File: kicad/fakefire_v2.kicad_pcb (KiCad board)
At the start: 2 copper layers, 212 x 96 mm, 46 parts, among them J1 Barrel_Jack, J2 Conn_01x03_Female, J3 Left speaker, J4 Right speaker, Q2 IRLB3813PBF, U1 YAAJ_DCDC_StepDown_LM2596, U2 PAM8403_Module, U3 TSOP1838B, U4 DFR0299, U5 Raspberry Pico, U6 4011

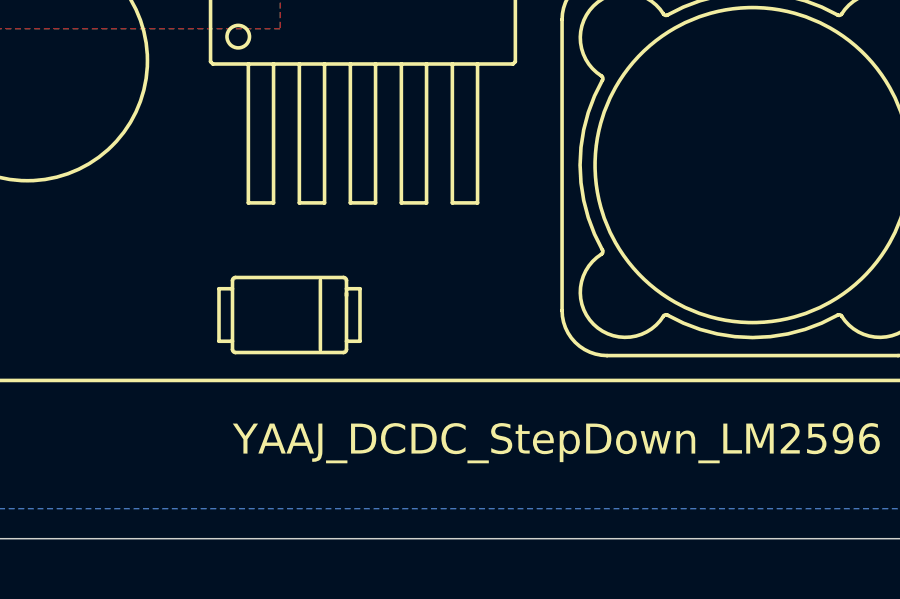
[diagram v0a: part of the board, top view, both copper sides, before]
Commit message: update kicad files, added more infos, comments
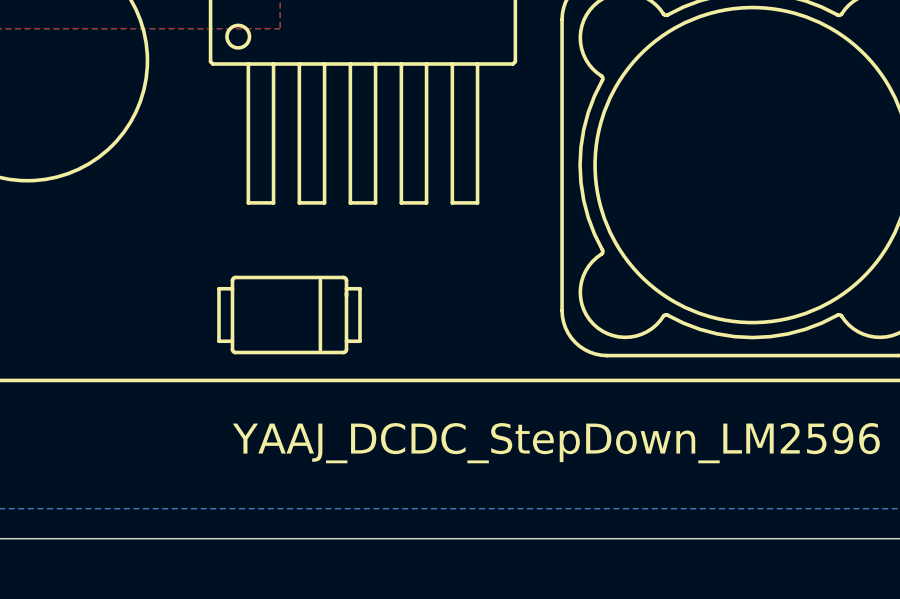
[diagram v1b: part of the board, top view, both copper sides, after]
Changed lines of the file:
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@@
   )
   (paper "A4")
+  (title_block
+    (title "Fakefire Project")
+    (date "2023-02-02")
+    (rev "1")
+    (company "N/A")
+  )
   (layers
     (0 "F.Cu" signal)
@@
     (fp_arc (start 20.467397 7.585796) (mid 20.906738 6.525137) (end 21.967397 6.085796) (layer "F.SilkS") (width 0.12))
     (fp_arc (start 21.781131 9.46601) (mid 21.825179 9.52623) (end 21.815218 9.600183) (layer "F.SilkS") (width 0.12))
-    (fp_arc (start 13.181636 16.183217) (mid 13.252353 16.212514) (end 13.281636 16.283217) (layer "F.SilkS") (width 0.12))
+    (fp_arc (start 13.181636 16.183217) (mid 13.252317 16.21252) (end 13.281636 16.283217) (layer "F.SilkS") (width 0.12))
     (fp_arc (start 13.281636 18.583217) (mid 13.252343 18.653929) (end 13.181636 18.683217) (layer "F.SilkS") (width 0.12))
-    (fp_arc (start 9.581636 18.683217) (mid 9.510931 18.653935) (end 9.481636 18.583217) (layer "F.SilkS") (width 0.12))
+    (fp_arc (start 9.581636 18.683217) (mid 9.510896 18.653941) (end 9.481636 18.583217) (layer "F.SilkS") (width 0.12))
     (fp_arc (start 23.981784 7.433617) (mid 26.817398 6.685796) (end 29.653011 7.433617) (layer "F.SilkS") (width 0.12))
     (fp_arc (start 21.815217 15.271409) (mid 21.825126 15.345337) (end 21.781132 15.405582) (layer "F.SilkS") (width 0.12))
@@
     (fp_arc (start 23.349783 3.632294) (mid 23.314441 3.617643) (end 23.299783 3.582294) (layer "F.SilkS") (width 0.12))
     (fp_arc (start 23.981783 7.433617) (mid 23.907854 7.443509) (end 23.847611 7.399531) (layer "F.SilkS") (width 0.12))
-    (fp_arc (start 23.847611 17.472062) (mid 23.907846 17.427997) (end 23.981783 17.437976) (layer "F.SilkS") (width 0.12))
+    (fp_arc (start 23.847611 17.472062) (mid 23.907831 17.428018) (end 23.981783 17.437976) (layer "F.SilkS") (width 0.12))
     (fp_arc (start 33.249783 -1.367705) (mid 33.285151 -1.353067) (end 33.299783 -1.317705) (layer "F.SilkS") (width 0.12))
     (fp_circle (center 26.817397 12.435796) (end 32.067397 12.435796) (layer "F.SilkS") (width 0.12) (fill none))
